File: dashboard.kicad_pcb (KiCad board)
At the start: 2 copper layers, 87.6 x 57.2 mm, 33 parts, among them J2 Conn_01x02, J3 RJ45, J4 Conn_01x10, J5 776267-1, Q1 2N7002, U1 TPS542025DDC, U2 R-78C5.0-1.0, U4 ILD74

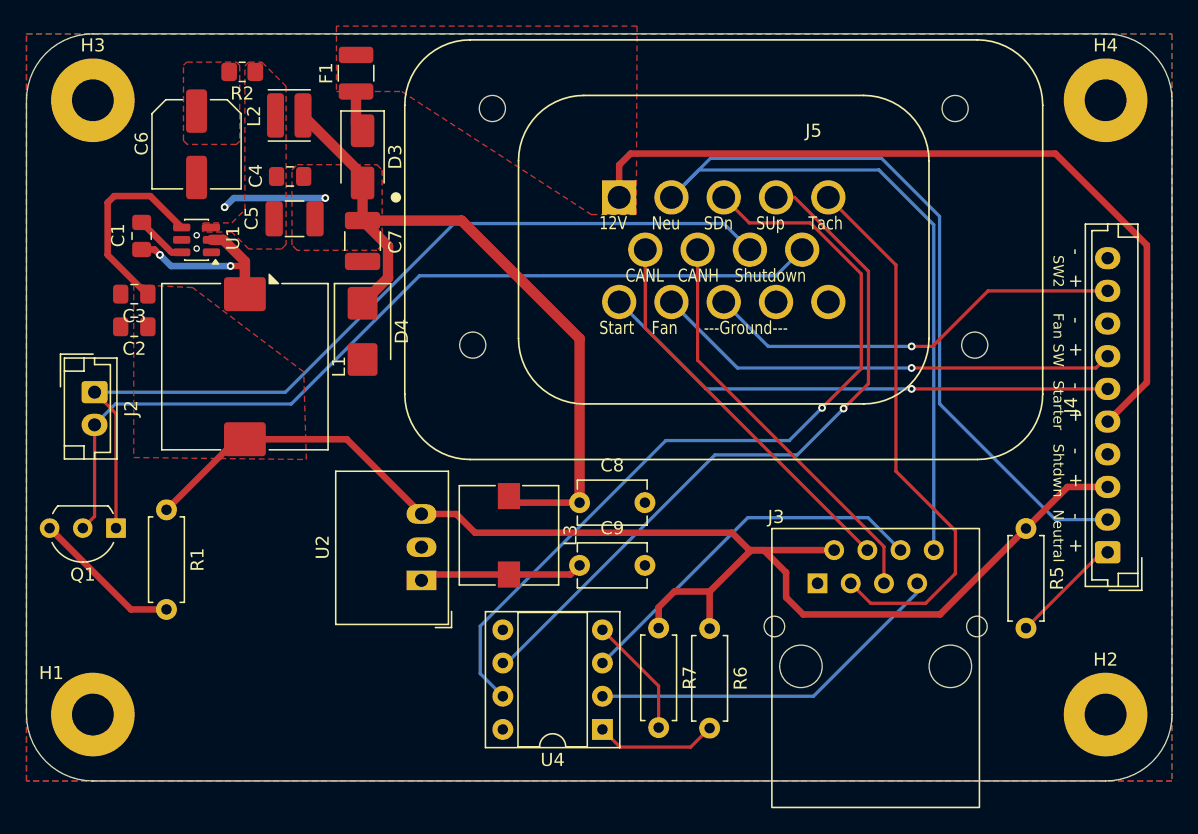
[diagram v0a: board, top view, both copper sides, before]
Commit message: Revert "added thermal vias for TPS54"
This reverts commit a34f3b064daca832ff572b55e7f0ad72ed936012.
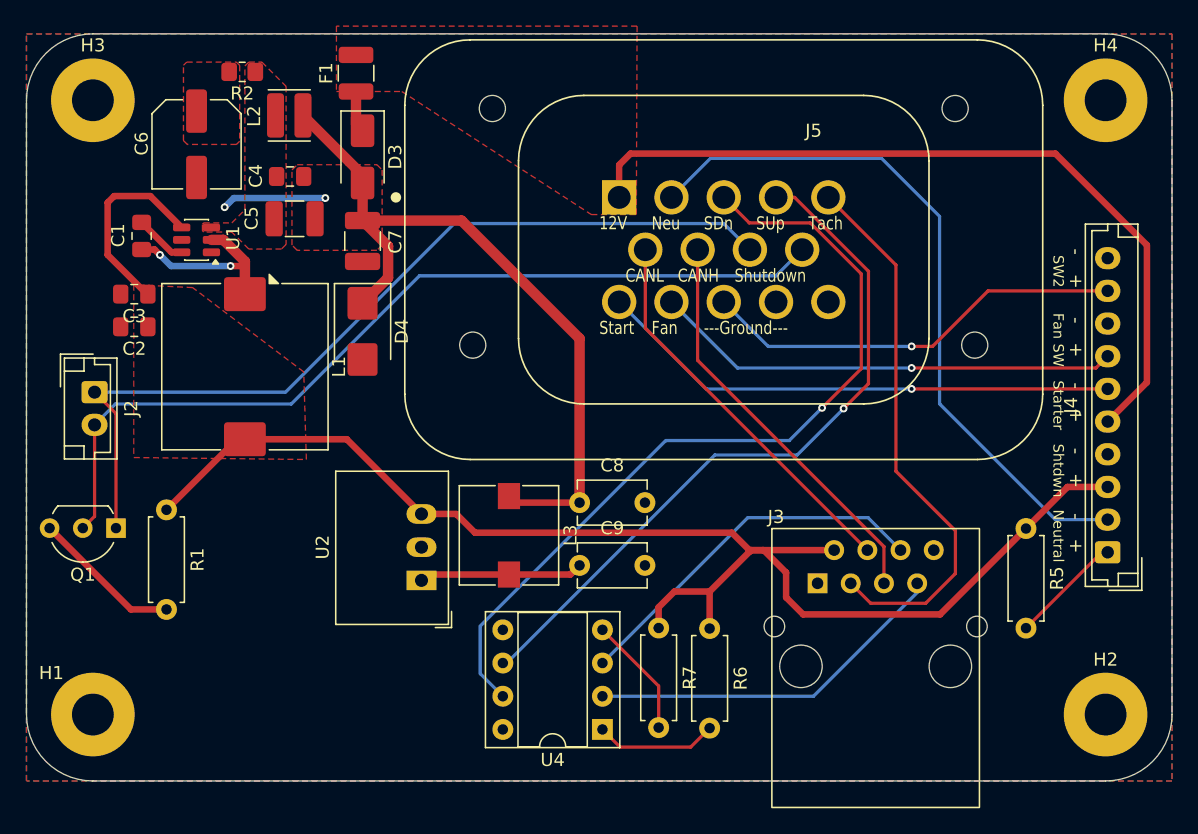
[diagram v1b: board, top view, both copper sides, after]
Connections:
- C1 pad 1: Net-(U1-VIN) -> Net-(U1-BOOT)
- C1 pad 2: Net-(C1-Pad2) -> Net-(U1-SW)
- C4 pad 1: Net-(U1-BOOT) -> Net-(U1-VIN)
- C5 pad 1: Net-(U1-BOOT) -> Net-(U1-VIN)
- L1 pad 1: Net-(C1-Pad2) -> Net-(U1-SW)
- L2 pad 2: Net-(U1-BOOT) -> Net-(U1-VIN)
- R2 pad 1: Net-(U1-BOOT) -> Net-(U1-VIN)
- U1 pad 2: unconnected-(U1-SW-Pad2) -> Net-(U1-SW)
- U1 pad 4: unconnected-(U1-FB-Pad4) -> +5V
- U1 pad 5: +5V -> unconnected-(U1-EN-Pad5)
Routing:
- net /Neutral: track 102.0 -> 54.4 mm
- net Net-(U1-SW): track 0.00 -> 14.3 mm, vias 0 -> 2
- net (no net): track 14.3 -> 0.00 mm, vias 2 -> 0
- net GND: vias 3 -> 2
- net +5V: vias 1 -> 0

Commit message: added thermal vias for TPS54
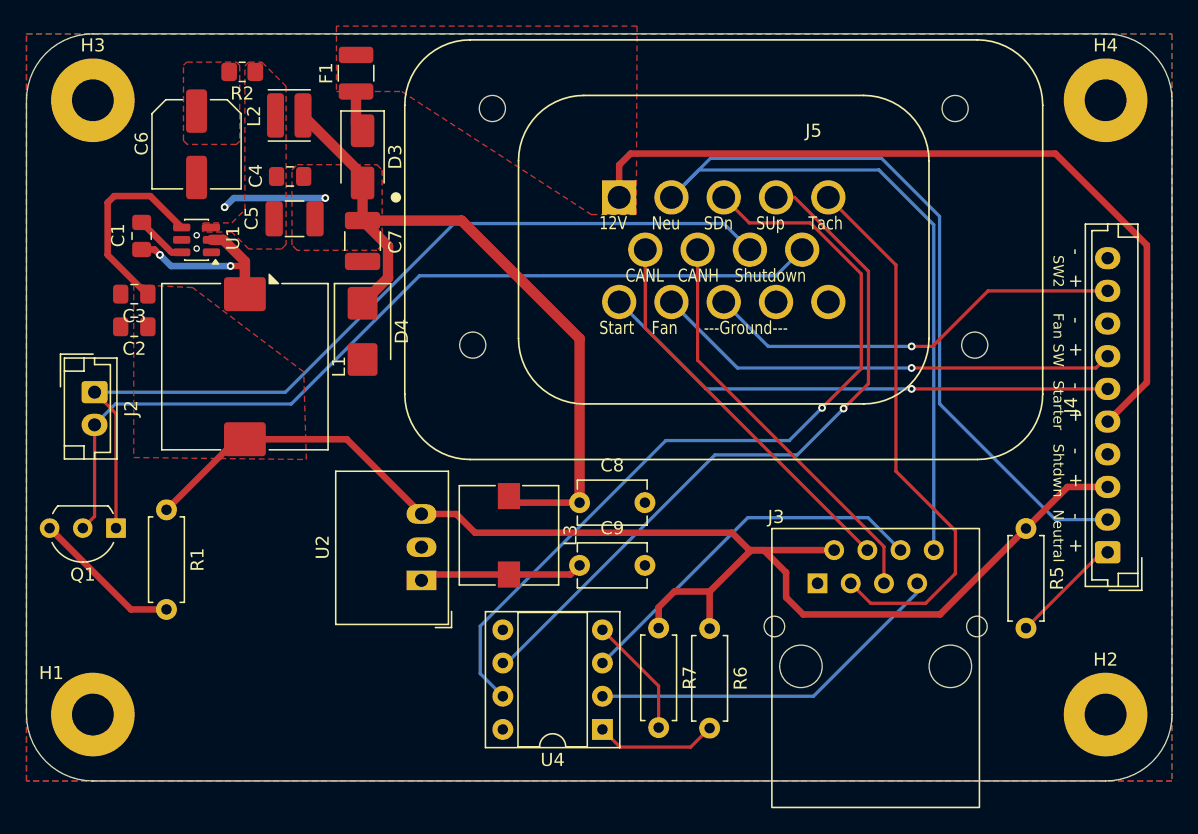
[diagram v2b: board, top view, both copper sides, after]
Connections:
- C1 pad 1: Net-(U1-BOOT) -> Net-(U1-VIN)
- C1 pad 2: Net-(U1-SW) -> Net-(C1-Pad2)
- C4 pad 1: Net-(U1-VIN) -> Net-(U1-BOOT)
- C5 pad 1: Net-(U1-VIN) -> Net-(U1-BOOT)
- L1 pad 1: Net-(U1-SW) -> Net-(C1-Pad2)
- L2 pad 2: Net-(U1-VIN) -> Net-(U1-BOOT)
- R2 pad 1: Net-(U1-VIN) -> Net-(U1-BOOT)
- U1 pad 2: Net-(U1-SW) -> unconnected-(U1-SW-Pad2)
- U1 pad 4: +5V -> unconnected-(U1-FB-Pad4)
- U1 pad 5: unconnected-(U1-EN-Pad5) -> +5V
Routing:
- net /Neutral: track 54.4 -> 102.0 mm
- net Net-(U1-SW): track 14.3 -> 0.00 mm, vias 2 -> 0
- net (no net): track 0.00 -> 14.3 mm, vias 0 -> 2
- net GND: vias 2 -> 3
- net +5V: vias 0 -> 1
